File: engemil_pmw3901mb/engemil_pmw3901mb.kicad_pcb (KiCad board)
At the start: 2 copper layers, 16 parts, among them J1 6130XX11121, U1 PMW3901MB-TXQT, U2 TLV77333PDBVR, U3 TLV77318PDBVR

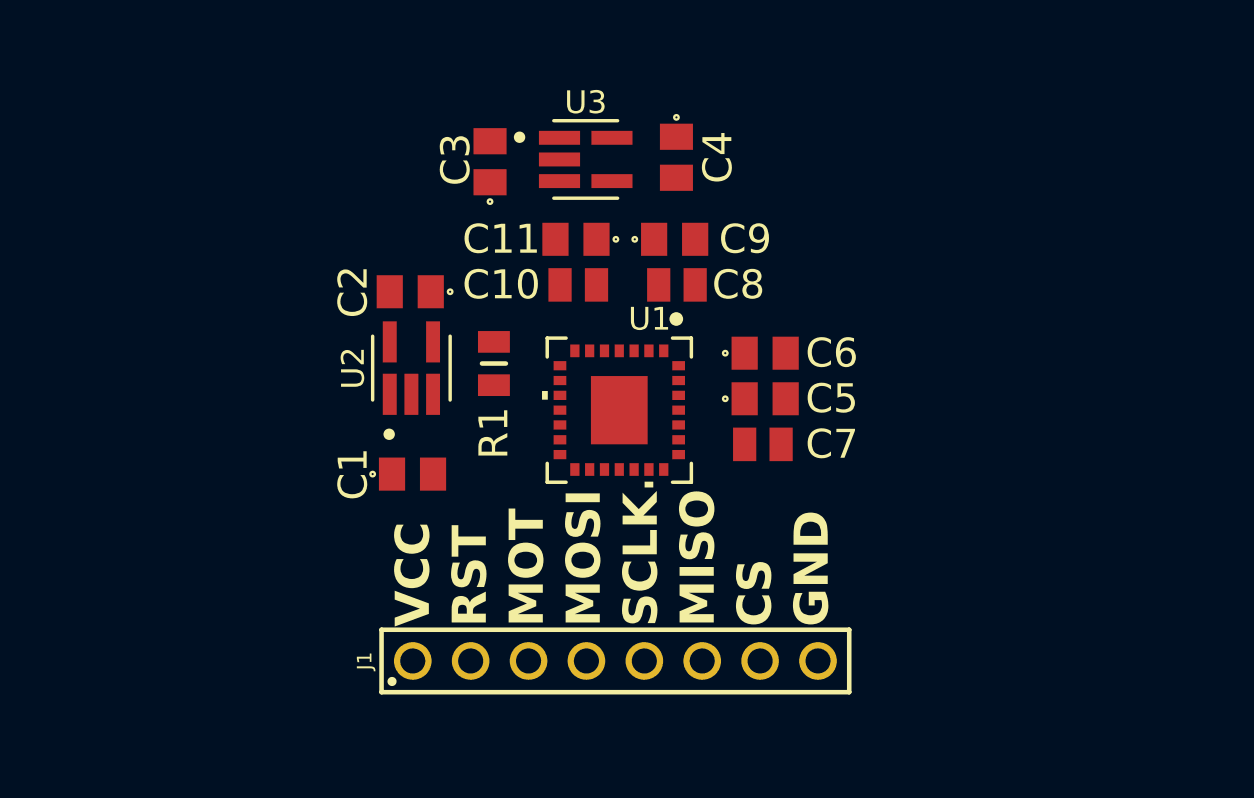
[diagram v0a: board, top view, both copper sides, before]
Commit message: Updated schematic and pcb
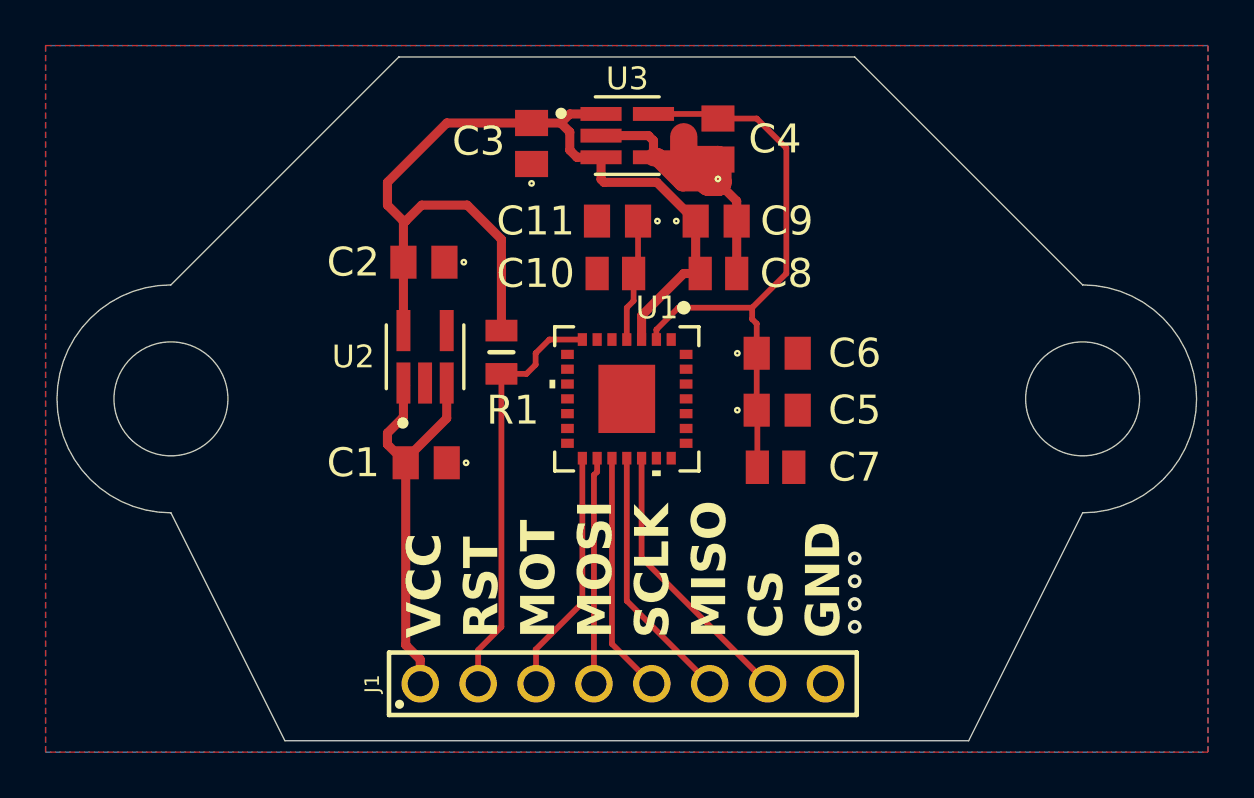
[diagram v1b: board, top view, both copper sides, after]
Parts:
- moved U3 2.10 mm to (150.0, 103.5)
- moved C4 1.99 mm to (154.0, 103.6), turned to 90 degrees
- moved C11 1.99 mm to (149.6, 107.2)
- moved C3 1.99 mm to (145.8, 103.8)
- moved C9 1.99 mm to (153.9, 107.2)
- moved C8 1.89 mm to (154.0, 109.5)
- moved C10 1.70 mm to (149.5, 109.5)
- moved C2 1.43 mm to (141.1, 109.0)
- moved C7 1.15 mm to (156.5, 118.0)
- moved J1 1.05 mm to (149.8, 127.5)
- moved C1 0.78 mm to (141.2, 117.8), turned to 180 degrees
- moved U2 0.78 mm to (141.1, 113.2)
- moved C5 0.73 mm to (156.6, 115.5)
- moved R1 0.60 mm to (144.5, 113.0)
- moved U1 0.60 mm to (150.0, 115.0)
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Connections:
- U1 pad 22: unconnected-(U1-NC-Pad22) -> GND
- U1 pad 23: unconnected-(U1-NC-Pad23) -> GND
- U1 pad 24: unconnected-(U1-NC-Pad24) -> GND
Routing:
- net +3.3V: track 0.00 -> 42.1 mm
- net +1V8: track 0.00 -> 26.2 mm
- net VCC: track 0.00 -> 19.0 mm
- net RESET: track 0.00 -> 18.5 mm
- net GND: track 0.00 -> 18.0 mm, vias 0 -> 4
- net CS: track 0.00 -> 12.2 mm
- net MISO: track 0.00 -> 11.4 mm
- net MOTION: track 0.00 -> 10.8 mm
- net SCLK: track 0.00 -> 10.6 mm
- net MOSI: track 0.00 -> 9.96 mm
- net Net-(U1-VREG): track 0.00 -> 5.40 mm
- added copper zone on B.Cu, net GND
- added copper zone on F.Cu, net GND
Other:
- board outline added: 50 x 30 mm
